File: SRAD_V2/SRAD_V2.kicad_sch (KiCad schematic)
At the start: 44 parts, among them SW1 SW_Push_Dual, SW2 SW_Nidec_CAS-120A1, U1 STM32F767ZIT6, U11 KX134-1211, U12 MAX-M10S, U13 MS5607-02BA, U14 MMC5983MA, U15 ASM330LHH, U16 MCP9808_DFN, U17 AS5F31G04SND-08LIN, U4 LSM6DSV80XTR

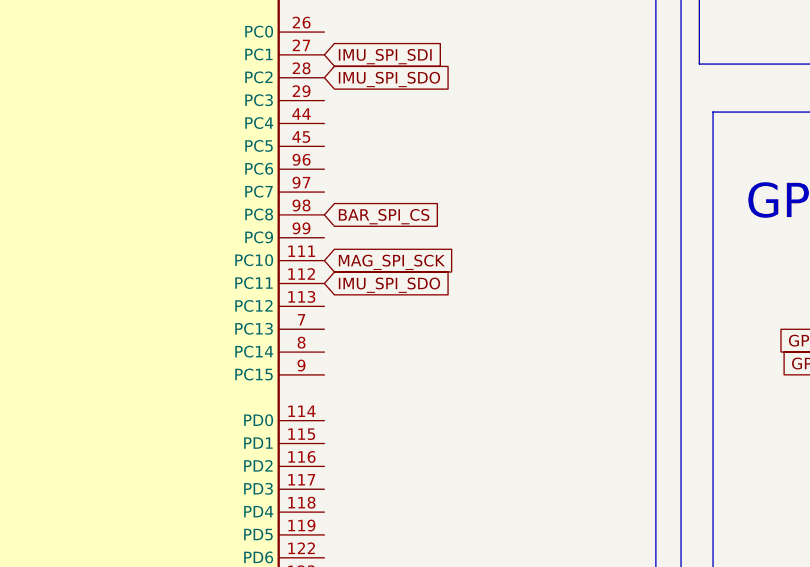
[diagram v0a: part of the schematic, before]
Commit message: Sensor routing and integration of various systems on the PCB
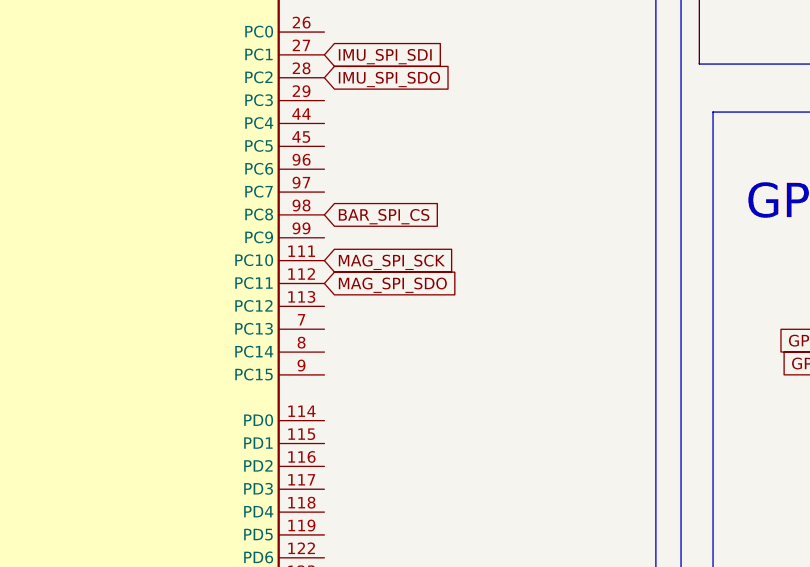
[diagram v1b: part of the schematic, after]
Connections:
- net IMU_SPI_SDO: no longer U1.112 (PC11)
- net MAG_SPI_SDO: now also U1.112 (PC11)
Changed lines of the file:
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@@
 		)
 	)
-	(global_label "IMU_SPI_SDO"
+	(global_label "MAG_SPI_SDO"
 		(shape input)
 		(at 118.11 205.74 0)
@@
 		)
 		(property "Intersheetrefs" "${INTERSHEET_REFS}"
-			(at 133.3114 205.74 0)
+			(at 133.7347 205.74 0)
 			(hide yes)
 			(show_name no)
